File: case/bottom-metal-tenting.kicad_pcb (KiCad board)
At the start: 2 copper layers, 148 x 100.4 mm, 10 parts

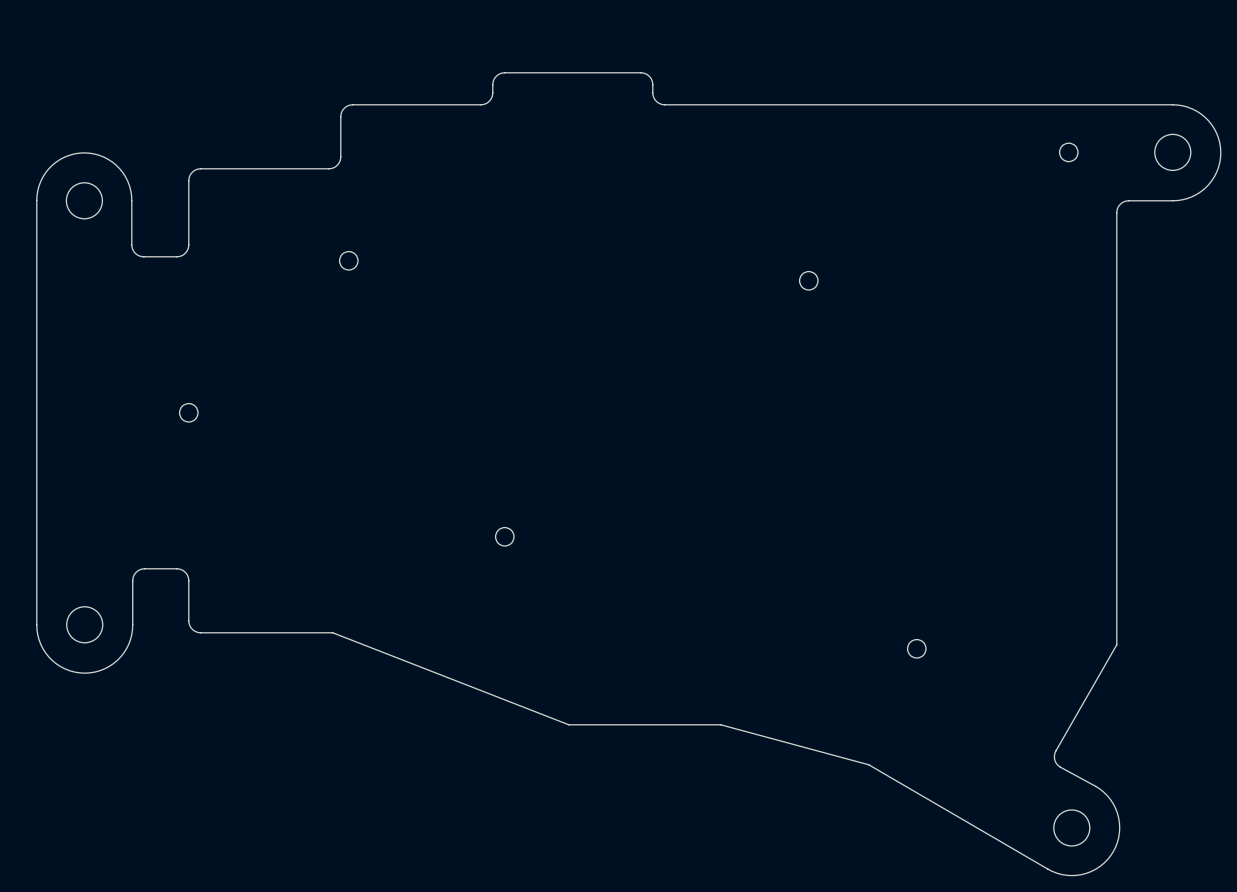
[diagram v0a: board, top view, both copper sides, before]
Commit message: update case files
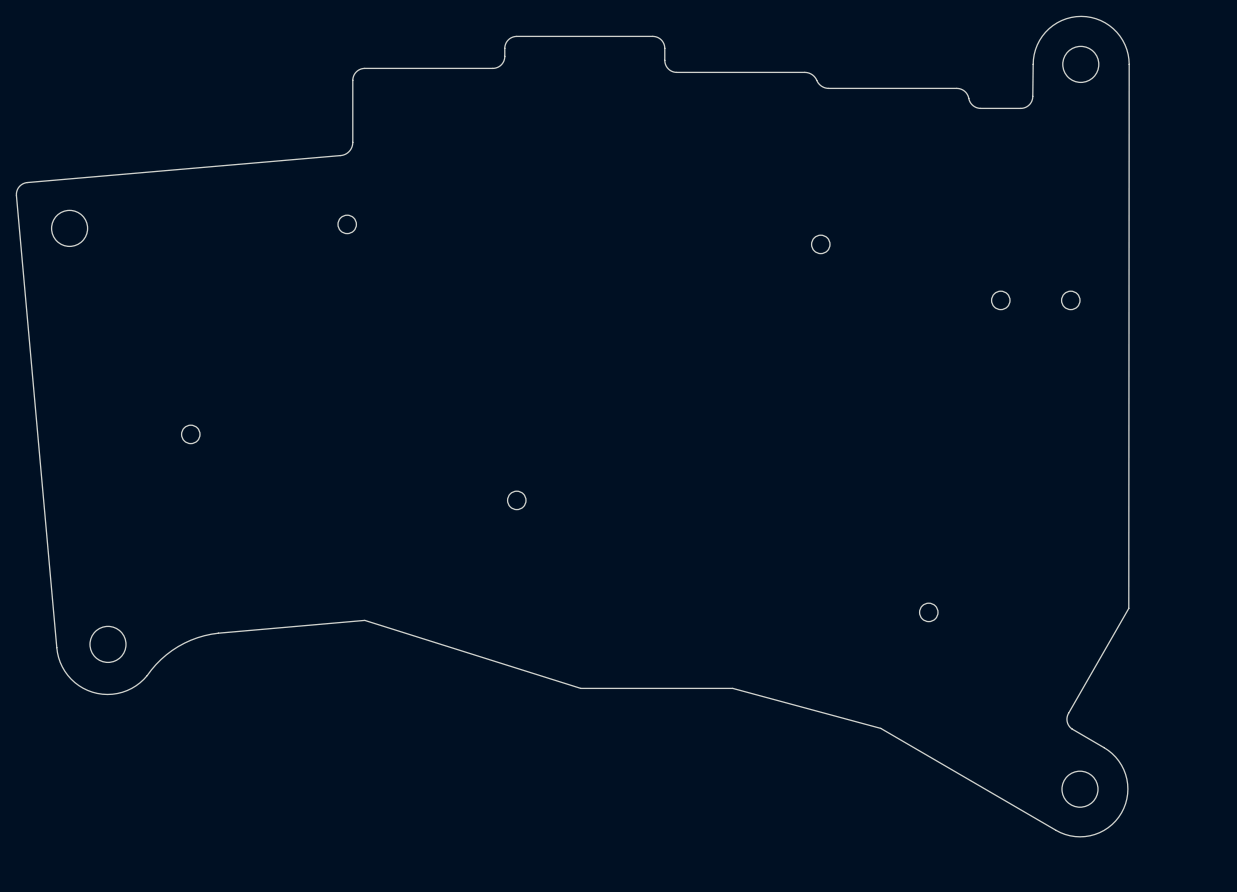
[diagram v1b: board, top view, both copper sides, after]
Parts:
- removed the H5 at (172.5, 74.0)
- removed the H5 at (205.0, 58.0)
- added H5: MountingHole, kbd:thread_m2, F.Cu at (174.0, 69.5)
- added H6: MountingHole, kbd:thread_m2, F.Cu at (196.5, 76.5)
- added H7: MountingHole, kbd:thread_m2, F.Cu at (205.2, 76.5)
- moved REF** 15.9 mm to (206.5, 47.0), turned to 90 degrees
- moved REF** 4.95 mm to (206.4, 137.6)
- moved H2 4.79 mm to (187.5, 115.5)
- moved H4 4.79 mm to (136.0, 101.5)
- moved H1 4.55 mm to (114.8, 67.0)
- moved REF** 3.92 mm to (80.1, 67.5), turned to 95 degrees
- moved REF** 3.80 mm to (84.9, 119.5), turned to -85 degrees
- moved H3 2.71 mm to (95.2, 93.2), turned to 5 degrees
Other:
- board size 148 x 100.4 mm -> 139.1 x 102.6 mm
